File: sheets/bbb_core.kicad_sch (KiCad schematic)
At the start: 11 parts, among them P10 BeagleBone_Black_Header, P11 BeagleBone_Black_Header, SW2 SW_DIP_x02, U2 CAT24C256

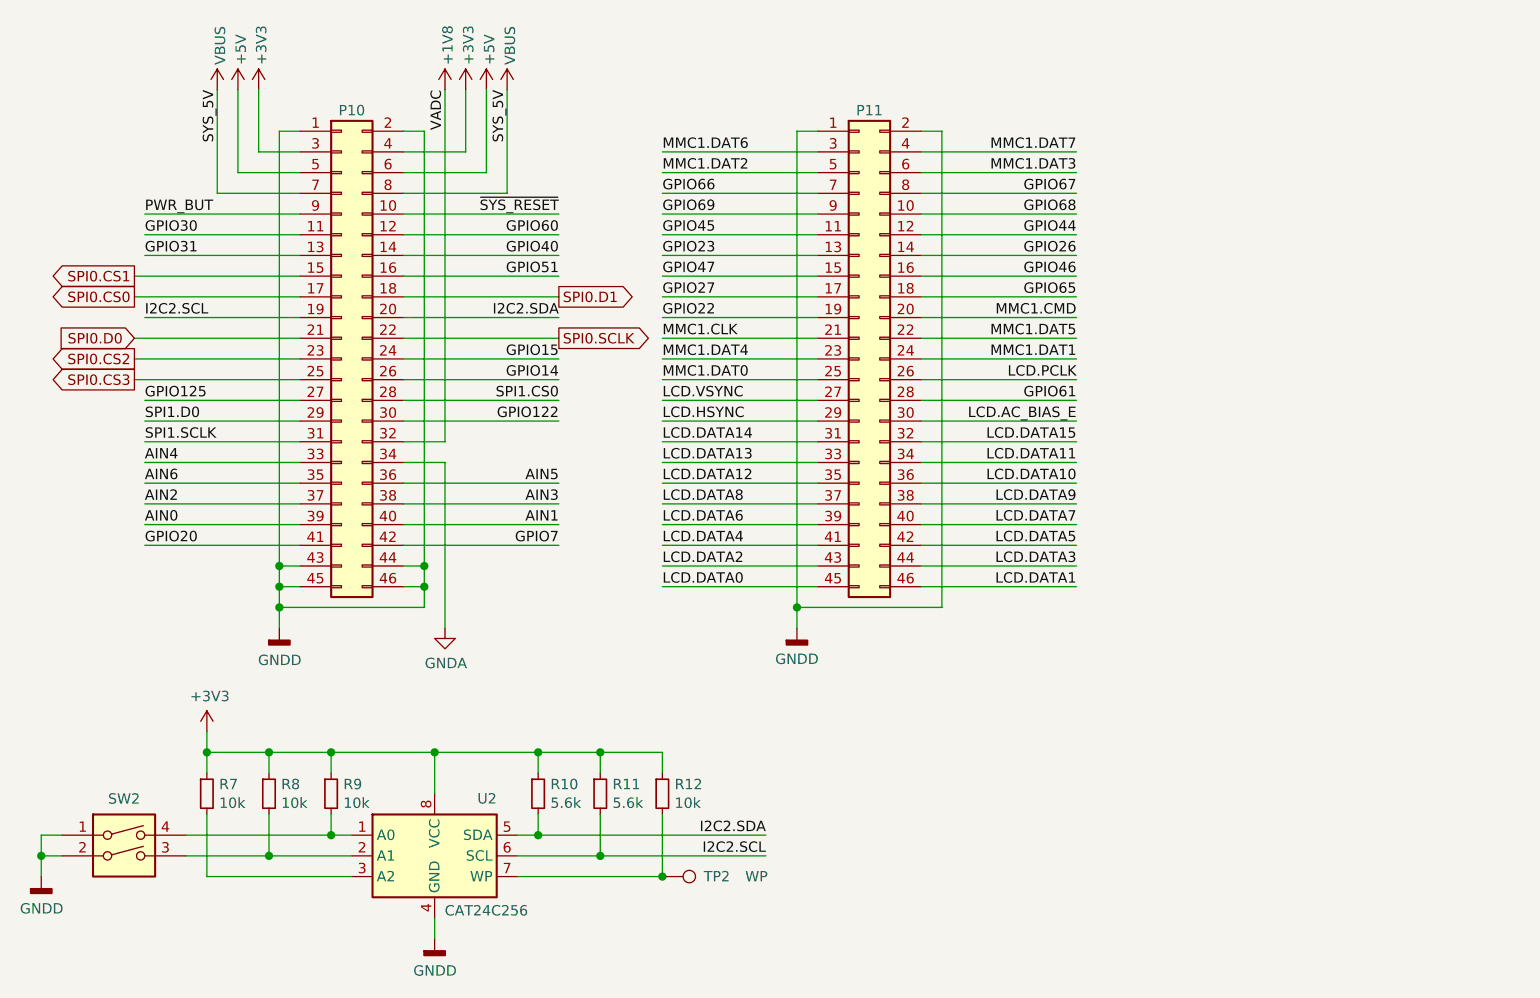
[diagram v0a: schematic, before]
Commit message: pushing storage
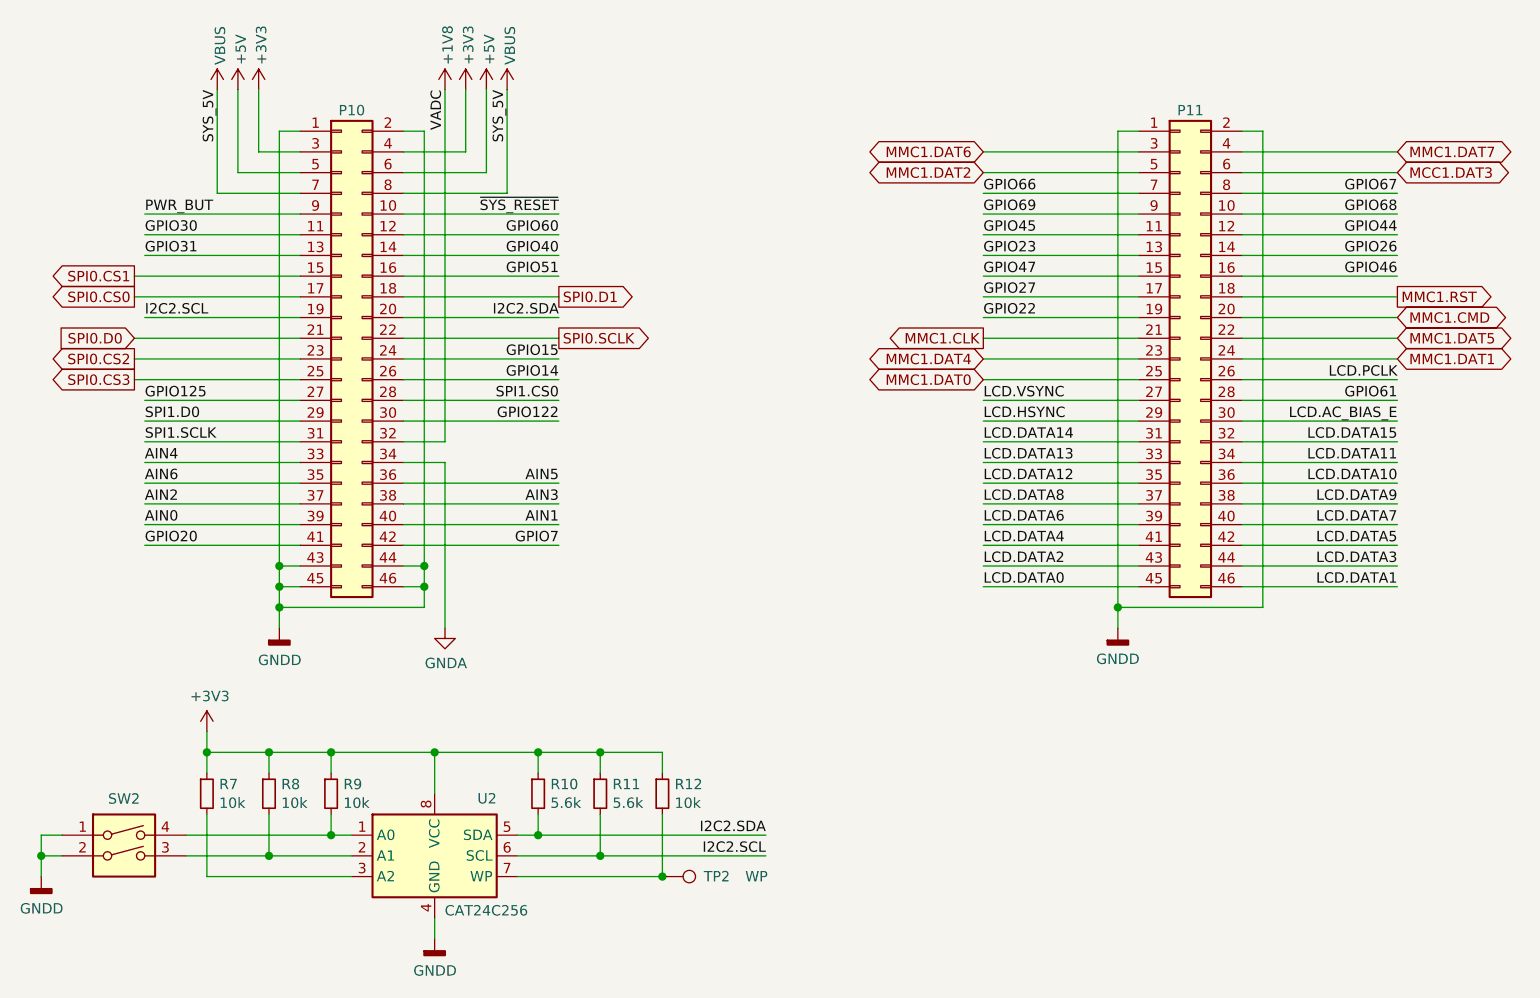
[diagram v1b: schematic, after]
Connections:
- net GPIO65 renamed MMC1.RST
- net MMC1.DAT3 renamed MCC1.DAT3
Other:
- moved on the sheet: P11

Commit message: push
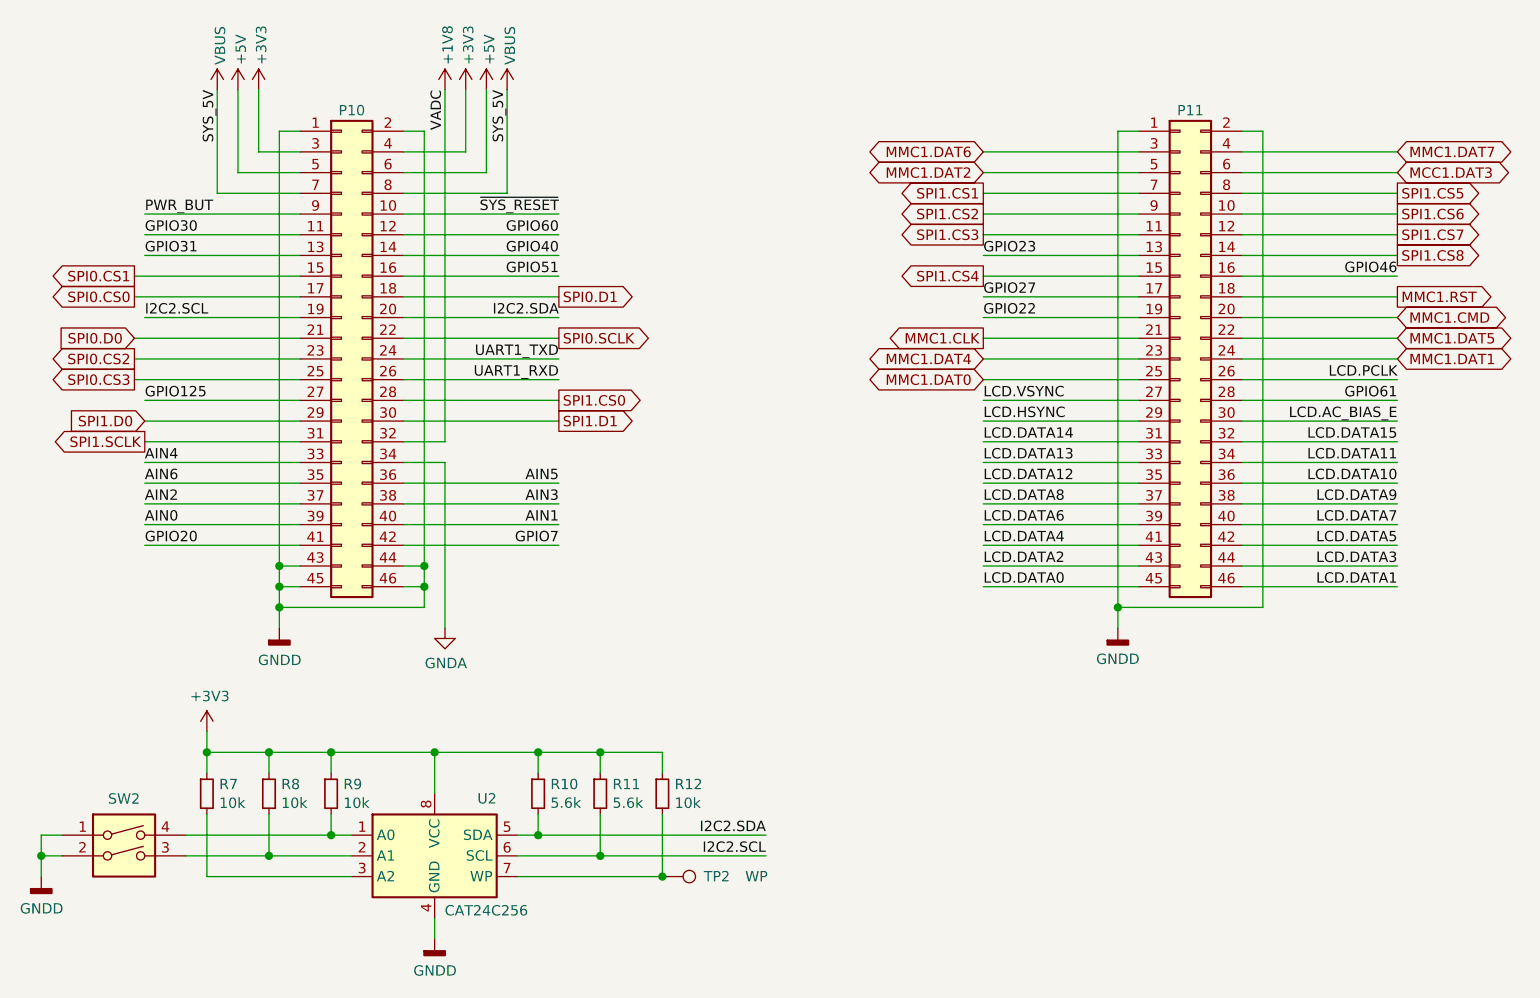
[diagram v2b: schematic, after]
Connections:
- net GPIO122 renamed SPI1.D1
- net GPIO14 renamed UART1_RXD
- net GPIO15 renamed UART1_TXD
- net GPIO26 renamed SPI1.CS8
- net GPIO44 renamed SPI1.CS7
- net GPIO45 renamed SPI1.CS3
- net GPIO47 renamed SPI1.CS4
- net GPIO66 renamed SPI1.CS1
- net GPIO67 renamed SPI1.CS5
- net GPIO68 renamed SPI1.CS6
- net GPIO69 renamed SPI1.CS2
